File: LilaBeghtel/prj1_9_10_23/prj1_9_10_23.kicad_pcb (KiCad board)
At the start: 2 copper layers, 7 parts, among them J1 Conn_01x04

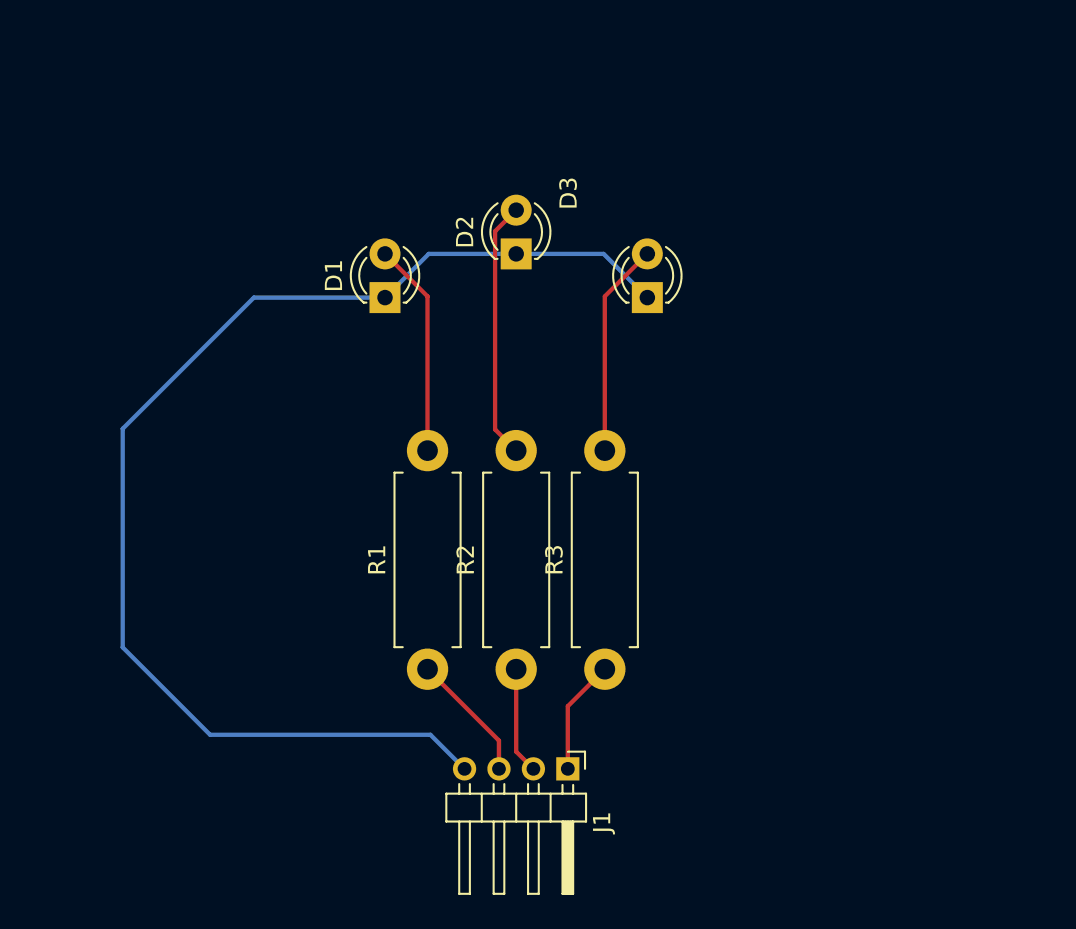
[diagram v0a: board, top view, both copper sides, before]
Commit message: new folder stuff
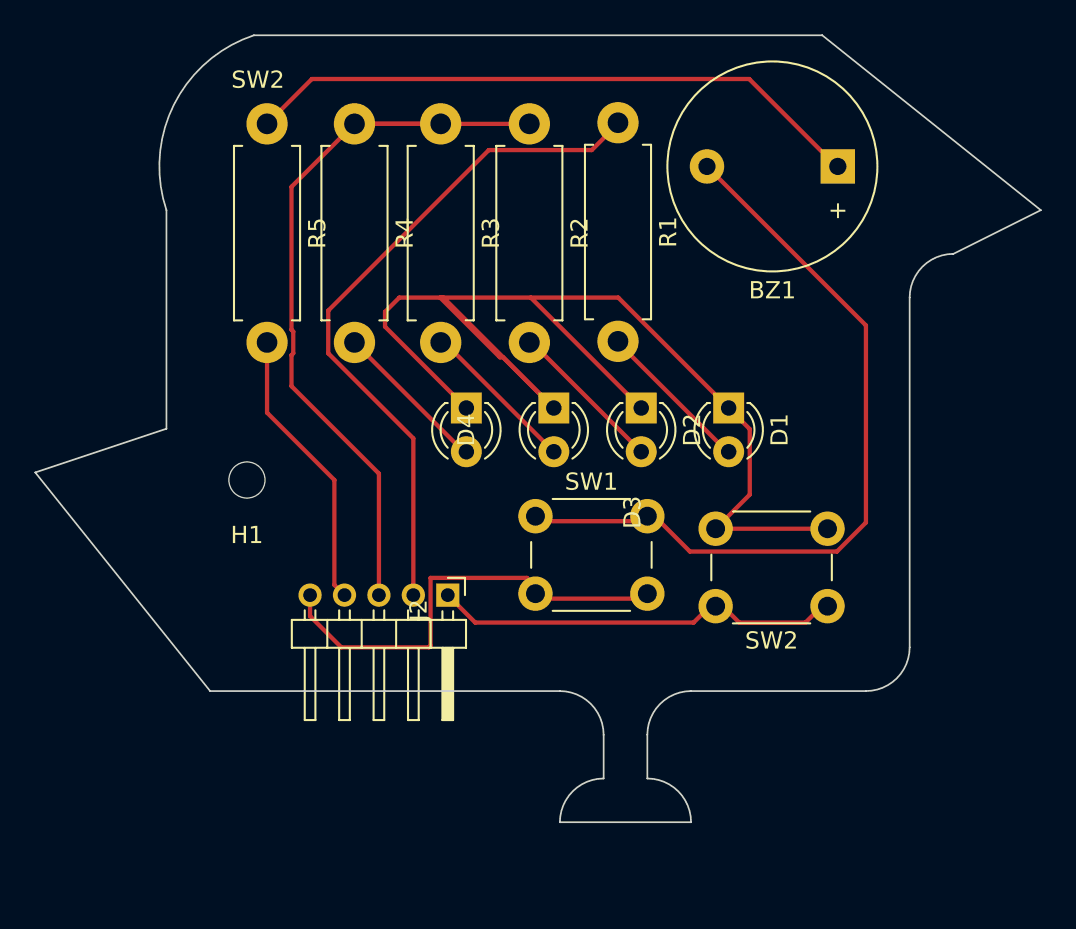
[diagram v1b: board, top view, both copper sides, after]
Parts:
- removed J1: Conn_01x04, Connector_PinHeader_2.00mm:PinHeader_1x04_P2.00mm_Horizontal
- added BZ1: Buzzer, Buzzer_Beeper:Buzzer_12x9.5RM7.6, F.Cu at (166.0, 73.7)
- added D4: LED, LED_THT:LED_D3.0mm, F.Cu at (144.4, 87.7)
- added H1: MountingHole, MountingHole:MountingHole_2.1mm, F.Cu at (131.7, 91.9)
- added J2: Conn_01x05_Pin, Connector_PinHeader_2.00mm:PinHeader_1x05_P2.00mm_Horizontal, F.Cu at (143.3, 98.6)
- added R4: R, Resistor_THT:R_Axial_DIN0411_L9.9mm_D3.6mm_P12.70mm_Horizontal, F.Cu at (137.9, 71.2)
- added R5: R, Resistor_THT:R_Axial_DIN0411_L9.9mm_D3.6mm_P12.70mm_Horizontal, F.Cu at (132.8, 71.2)
- added SW1: SW_Push_Open, Button_Switch_THT:SW_PUSH_6mm, F.Cu at (148.4, 94.0)
- added SW2: SW_Push_Open, Button_Switch_THT:SW_PUSH_6mm, F.Cu at (165.4, 99.2)
- moved R1 33.6 mm to (153.2, 71.1), turned to -90 degrees
- moved R3 33.1 mm to (142.9, 71.2), turned to -90 degrees
- moved R2 31.7 mm to (148.1, 71.2), turned to -90 degrees
- moved D1 21.0 mm to (159.7, 87.7), turned to -90 degrees
- moved D2 11.5 mm to (154.6, 87.7), turned to -90 degrees
- moved D3 8.41 mm to (149.5, 87.7), turned to -90 degrees
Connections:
- R2 pad 1: Net-(J1-Pin_2) -> Net-(J2-Pin_3)
- R3 pad 1: Net-(J1-Pin_1) -> Net-(J2-Pin_3)
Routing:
- net Net-(J2-Pin_3): track 0.00 -> 46.4 mm
- net Net-(BZ1-+): track 0.00 -> 44.4 mm
- net Net-(BZ1--): track 0.00 -> 36.4 mm
- net Net-(J2-Pin_2): track 7.51 -> 39.9 mm
- net Net-(J2-Pin_5): track 0.00 -> 26.8 mm
- net Net-(J2-Pin_1): track 0.00 -> 24.4 mm
- net Net-(J2-Pin_4): track 0.00 -> 16.5 mm
- net Net-(D4-A): track 0.00 -> 9.13 mm
- net Net-(J1-Pin_1): track 6.68 -> 0.00 mm
- net Net-(J1-Pin_2): track 6.20 -> 0.00 mm
- net Net-(D2-A): track 15.0 -> 9.28 mm
- net Net-(D1-A): track 12.5 -> 9.06 mm
- net Net-(D3-A): track 12.5 -> 9.42 mm
- net Net-(D1-K): track 71.2 -> 73.4 mm
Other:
- board outline added: 58.4 x 45.7 mm
- board text added: "SW2"
- board text added: "SW_Push_Open"
